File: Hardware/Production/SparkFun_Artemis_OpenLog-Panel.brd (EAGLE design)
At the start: 106.2 x 205 mm, 2031 parts, among them J100 CORTEX_JTAG, J107 MICRO-SD, J109 CORTEX_JTAG, J116 MICRO-SD, J118 CORTEX_JTAG, J125 MICRO-SD, J127 CORTEX_JTAG, J134 MICRO-SD, J14 CORTEX_JTAG, J17 MICRO-SD, J19 CORTEX_JTAG, J26 MICRO-SD, J28 CORTEX_JTAG, J35 MICRO-SD, J37 CORTEX_JTAG, J44 MICRO-SD, J46 CORTEX_JTAG, J53 MICRO-SD, J55 CORTEX_JTAG, J6 MICRO-SD, J62 MICRO-SD, J64 CORTEX_JTAG, J71 MICRO-SD, J73 CORTEX_JTAG, J8 CORTEX_JTAG, J80 MICRO-SD, J82 CORTEX_JTAG, J89 MICRO-SD, J91 CORTEX_JTAG, J98 MICRO-SD, Q1 20V/0.2A/8MHz/1.2Ω/1Vth, Q10 20V/0.2A/8MHz/1.2Ω/1Vth, Q11 20V/0.2A/8MHz/1.2Ω/1Vth, Q12 20V/4.2A/52mΩ/1.4W, Q13 20V/0.2A/8MHz/1.2Ω/1Vth, Q14 20V/0.2A/8MHz/1.2Ω/1Vth, Q15 20V/0.2A/8MHz/1.2Ω/1Vth, Q16 20V/0.2A/8MHz/1.2Ω/1Vth, Q17 20V/0.2A/8MHz/1.2Ω/1Vth, Q18 20V/4.2A/52mΩ/1.4W, Q19 20V/0.2A/8MHz/1.2Ω/1Vth, Q2 20V/4.2A/52mΩ/1.4W, Q20 20V/0.2A/8MHz/1.2Ω/1Vth, Q21 20V/0.2A/8MHz/1.2Ω/1Vth, Q22 20V/0.2A/8MHz/1.2Ω/1Vth, Q23 20V/0.2A/8MHz/1.2Ω/1Vth, Q24 20V/4.2A/52mΩ/1.4W, Q25 20V/0.2A/8MHz/1.2Ω/1Vth, Q26 20V/0.2A/8MHz/1.2Ω/1Vth, Q27 20V/0.2A/8MHz/1.2Ω/1Vth, Q28 20V/0.2A/8MHz/1.2Ω/1Vth, Q29 20V/0.2A/8MHz/1.2Ω/1Vth, Q3 20V/0.2A/8MHz/1.2Ω/1Vth, Q30 20V/4.2A/52mΩ/1.4W, Q31 20V/0.2A/8MHz/1.2Ω/1Vth, Q32 20V/0.2A/8MHz/1.2Ω/1Vth, Q33 20V/0.2A/8MHz/1.2Ω/1Vth, Q34 20V/0.2A/8MHz/1.2Ω/1Vth, Q35 20V/0.2A/8MHz/1.2Ω/1Vth, Q36 20V/4.2A/52mΩ/1.4W, Q37 20V/0.2A/8MHz/1.2Ω/1Vth, Q38 20V/0.2A/8MHz/1.2Ω/1Vth, Q39 20V/0.2A/8MHz/1.2Ω/1Vth, Q4 20V/0.2A/8MHz/1.2Ω/1Vth, Q40 20V/0.2A/8MHz/1.2Ω/1Vth, Q41 20V/0.2A/8MHz/1.2Ω/1Vth, Q42 20V/4.2A/52mΩ/1.4W, Q43 20V/0.2A/8MHz/1.2Ω/1Vth, Q44 20V/0.2A/8MHz/1.2Ω/1Vth, Q45 20V/0.2A/8MHz/1.2Ω/1Vth, Q46 20V/0.2A/8MHz/1.2Ω/1Vth, Q47 20V/0.2A/8MHz/1.2Ω/1Vth, Q48 20V/4.2A/52mΩ/1.4W, Q49 20V/0.2A/8MHz/1.2Ω/1Vth, Q5 20V/0.2A/8MHz/1.2Ω/1Vth, Q50 20V/0.2A/8MHz/1.2Ω/1Vth, Q51 20V/0.2A/8MHz/1.2Ω/1Vth, Q52 20V/0.2A/8MHz/1.2Ω/1Vth, Q53 20V/0.2A/8MHz/1.2Ω/1Vth, Q54 20V/4.2A/52mΩ/1.4W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

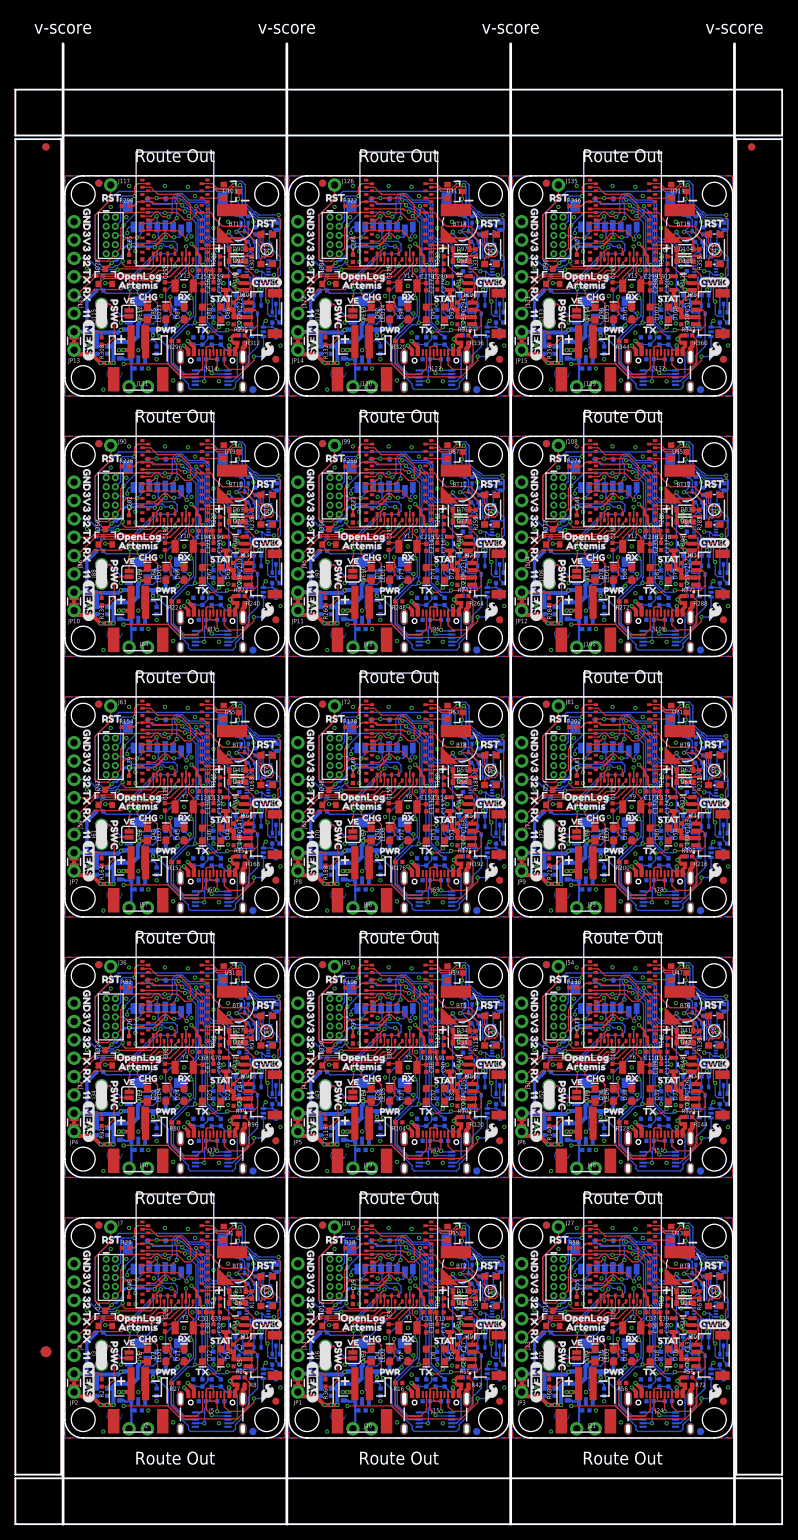
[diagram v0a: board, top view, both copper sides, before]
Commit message: Final V10 PCB tweaks!?
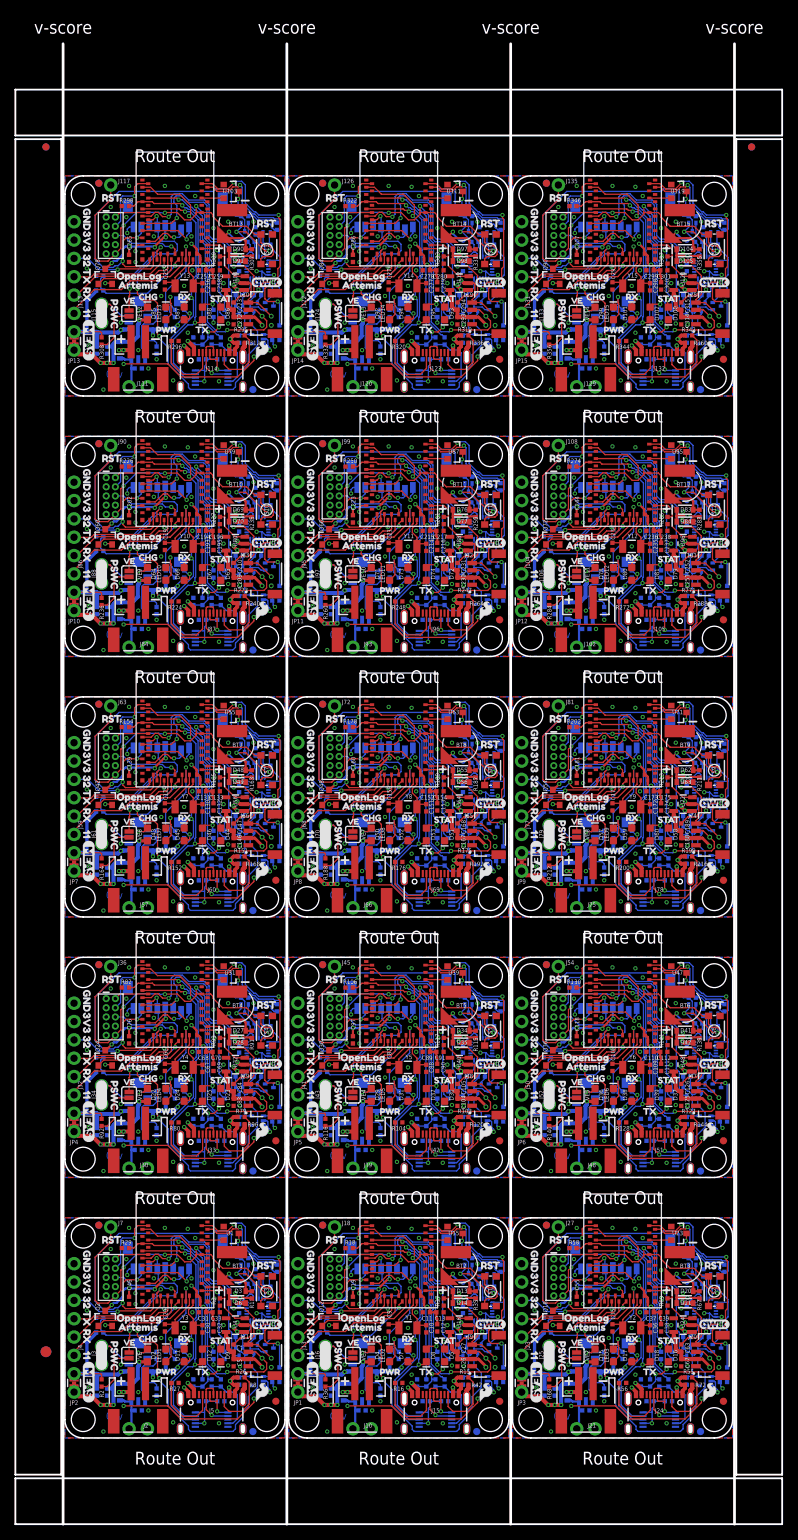
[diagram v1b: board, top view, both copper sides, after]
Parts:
- added GND, GND1, GND10, GND11, GND12, GND13, GND14, GND2, GND3, GND4, GND5, GND6, GND7, GND8, GND9, QWIIC_3.3V, QWIIC_3.3V1, QWIIC_3.3V10, QWIIC_3.3V11, QWIIC_3.3V12, QWIIC_3.3V13, QWIIC_3.3V14, QWIIC_3.3V2, QWIIC_3.3V3, QWIIC_3.3V4, QWIIC_3.3V5, QWIIC_3.3V6, QWIIC_3.3V7, QWIIC_3.3V8, QWIIC_3.3V9: TEST-POINTTP_15TH_THRU, SparkFun-Connectors:TP_15TH
- added U$586: (no value), buzzard_labels (14):322
- added U$587, U$588: (no value), buzzard_labels (14):GND5
- added U$589, U$590: (no value), buzzard_labels (14):RX1
- added U$591, U$592: (no value), buzzard_labels (14):TX0
- added U$593, U$594: (no value), buzzard_labels:PSWC0
- added U$595: (no value), buzzard_labels (19):VE0
- added U$596, U$597: (no value), RST_04:RST0
- added U$598: (no value), output:C0
- added U$599: (no value), output:D0
- added U$600: (no value), output:30
- SCL, SCL1, SCL10, SCL11, SCL12, SCL13, SCL14, SCL2, SCL3, SCL4, SCL5, SCL6, SCL7, SCL8, SCL9, SDA, SDA1, SDA10, SDA11, SDA12, SDA13, SDA14, SDA2, SDA3, SDA4, SDA5, SDA6, SDA7, SDA8, SDA9: value TEST-POINT3 -> TEST-POINTTP_15TH_THRU; device SparkFun-Connectors:PAD.03X.03 -> SparkFun-Connectors:TP_15TH
- U$100, U$60: device buzzard_labels (14):3V34 -> buzzard_labels (13):VIN8
- U$101, U$102, U$141, U$62: device buzzard_labels (14):113 -> buzzard_labels (14):3V34
- U$103, U$104, U$143, U$64: device buzzard_labels (14):322 -> buzzard_labels (14):113
- U$105, U$106, U$145, U$66: device buzzard_labels (14):GND5 -> buzzard_labels (14):322
- U$107, U$108, U$147, U$68: device buzzard_labels (14):RX1 -> buzzard_labels (14):GND5
- U$109, U$110, U$149, U$70: device buzzard_labels (14):TX0 -> buzzard_labels (14):RX1
- U$111, U$112, U$151, U$72: device buzzard_labels:PSWC0 -> buzzard_labels (14):TX0
- U$113, U$74: device buzzard_labels (19):VE0 -> buzzard_labels:PSWC0
- U$114, U$153, U$154, U$193: device RST_04:RST0 -> buzzard_labels:PSWC0
- U$115, U$75: device RST_04:RST0 -> buzzard_labels (19):VE0
- U$116, U$77: device output:C0 -> RST_04:RST0
- U$117, U$156: device output:D0 -> RST_04:RST0
- U$118: device buzzard_labels (2):MEAS3 -> output:C0
- U$119, U$359: device buzzard_labels (1):X0 -> output:D0
- U$120, U$360: device buzzard_labels (1):Y1 -> output:30
- U$121, U$361: device buzzard_labels (1):Z2 -> buzzard_labels (2):MEAS3
- U$122: device buzzard_labels (1):G5 -> buzzard_labels (1):X0
- U$123: device buzzard_labels (1):A4 -> buzzard_labels (1):Y1
- U$124: device buzzard_labels (1):M3 -> buzzard_labels (1):Z2
- U$125: device buzzard_labels (1):X0 -> buzzard_labels (1):G5
- U$126: device buzzard_labels (1):Y1 -> buzzard_labels (1):A4
- U$127: device buzzard_labels (1):Z2 -> buzzard_labels (1):M3
- U$128, U$362: device qwiic#logo#jpg:QWIIC#LOGO#JPG -> buzzard_labels (1):X0
- U$129, U$363: device buzzard_labels (12):CHG2 -> buzzard_labels (1):Y1
- U$130, U$364: device buzzard_labels (12):PWR0 -> buzzard_labels (1):Z2
- U$131: device buzzard_labels (12):RX4 -> qwiic#logo#jpg:QWIIC#LOGO#JPG
- U$132: device buzzard_labels (12):STAT5 -> buzzard_labels (12):CHG2
- U$133: device buzzard_labels (12):TX3 -> buzzard_labels (12):PWR0
- U$134: device buzzard_labels (13):ARTEMIS13 -> buzzard_labels (12):RX4
- U$135: device buzzard_labels (13):OPENLOG12 -> buzzard_labels (12):STAT5
- U$136: device buzzard_labels (13):RST9 -> buzzard_labels (12):TX3
- U$137: device buzzard_labels (13):VIN8 -> buzzard_labels (13):ARTEMIS13
- U$138, U$178: device buzzard_labels (14):3V34 -> buzzard_labels (13):OPENLOG12
- U$139, U$99: device buzzard_labels (14):3V34 -> buzzard_labels (13):RST9
- U$140, U$180: device buzzard_labels (14):113 -> buzzard_labels (13):VIN8
- U$142, U$181, U$182, U$221: device buzzard_labels (14):322 -> buzzard_labels (14):3V34
- U$144, U$183, U$184, U$223: device buzzard_labels (14):GND5 -> buzzard_labels (14):113
- U$146, U$185, U$186, U$225: device buzzard_labels (14):RX1 -> buzzard_labels (14):322
- U$148, U$187, U$188, U$227: device buzzard_labels (14):TX0 -> buzzard_labels (14):GND5
- U$15: device buzzard_labels (2):MEAS3 -> output:30
- U$150, U$189, U$190, U$229: device buzzard_labels:PSWC0 -> buzzard_labels (14):RX1
- U$152, U$191: device buzzard_labels (19):VE0 -> buzzard_labels (14):TX0
- U$155: device output:C0 -> buzzard_labels (19):VE0
- U$157, U$196: device buzzard_labels (2):MEAS3 -> RST_04:RST0
- U$158, U$398: device buzzard_labels (1):X0 -> output:C0
- U$159, U$399: device buzzard_labels (1):Y1 -> output:D0
- U$16, U$281: device buzzard_labels (1):X0 -> buzzard_labels (2):MEAS3
- U$160, U$400: device buzzard_labels (1):Z2 -> output:30
- U$161: device buzzard_labels (1):G5 -> buzzard_labels (2):MEAS3
- U$162: device buzzard_labels (1):A4 -> buzzard_labels (1):X0
- U$163: device buzzard_labels (1):M3 -> buzzard_labels (1):Y1
- U$164: device buzzard_labels (1):X0 -> buzzard_labels (1):Z2
- U$165: device buzzard_labels (1):Y1 -> buzzard_labels (1):G5
- U$166: device buzzard_labels (1):Z2 -> buzzard_labels (1):A4
- U$167: device qwiic#logo#jpg:QWIIC#LOGO#JPG -> buzzard_labels (1):M3
- U$168, U$402: device buzzard_labels (12):CHG2 -> buzzard_labels (1):X0
- U$169, U$403: device buzzard_labels (12):PWR0 -> buzzard_labels (1):Y1
- U$17, U$23, U$282: device buzzard_labels (1):Y1 -> buzzard_labels (1):X0
- U$170, U$404: device buzzard_labels (12):RX4 -> buzzard_labels (1):Z2
- U$171: device buzzard_labels (12):STAT5 -> qwiic#logo#jpg:QWIIC#LOGO#JPG
- U$172: device buzzard_labels (12):TX3 -> buzzard_labels (12):CHG2
- U$173: device buzzard_labels (13):ARTEMIS13 -> buzzard_labels (12):PWR0
- U$174: device buzzard_labels (13):OPENLOG12 -> buzzard_labels (12):RX4
- U$175: device buzzard_labels (13):RST9 -> buzzard_labels (12):STAT5
- U$176: device buzzard_labels (13):VIN8 -> buzzard_labels (12):TX3
- U$177, U$217: device buzzard_labels (14):3V34 -> buzzard_labels (13):ARTEMIS13
- U$179, U$219: device buzzard_labels (14):113 -> buzzard_labels (13):RST9
- U$18, U$24, U$283: device buzzard_labels (1):Z2 -> buzzard_labels (1):Y1
- U$19: device buzzard_labels (1):G5 -> buzzard_labels (1):Z2
- U$192, U$231, U$232, U$271: device RST_04:RST0 -> buzzard_labels (14):TX0
- U$194, U$233: device output:C0 -> buzzard_labels:PSWC0
- U$195: device output:D0 -> buzzard_labels (19):VE0
- U$197, U$236, U$437, U$476: device buzzard_labels (1):X0 -> RST_04:RST0
- U$198, U$438: device buzzard_labels (1):Y1 -> output:C0
- U$199, U$439: device buzzard_labels (1):Z2 -> output:D0
- U$20: device buzzard_labels (1):A4 -> buzzard_labels (1):G5
- U$200: device buzzard_labels (1):G5 -> output:30
- U$201: device buzzard_labels (1):A4 -> buzzard_labels (2):MEAS3
- U$202: device buzzard_labels (1):M3 -> buzzard_labels (1):X0
- U$203: device buzzard_labels (1):X0 -> buzzard_labels (1):Y1
- U$204: device buzzard_labels (1):Y1 -> buzzard_labels (1):Z2
- U$205: device buzzard_labels (1):Z2 -> buzzard_labels (1):G5
- U$206: device qwiic#logo#jpg:QWIIC#LOGO#JPG -> buzzard_labels (1):A4
- U$207: device buzzard_labels (12):CHG2 -> buzzard_labels (1):M3
- U$208, U$442: device buzzard_labels (12):PWR0 -> buzzard_labels (1):X0
- U$209, U$443: device buzzard_labels (12):RX4 -> buzzard_labels (1):Y1
- U$21: device buzzard_labels (1):M3 -> buzzard_labels (1):A4
- U$210, U$444: device buzzard_labels (12):STAT5 -> buzzard_labels (1):Z2
- U$211: device buzzard_labels (12):TX3 -> qwiic#logo#jpg:QWIIC#LOGO#JPG
- U$212: device buzzard_labels (13):ARTEMIS13 -> buzzard_labels (12):CHG2
- U$213: device buzzard_labels (13):OPENLOG12 -> buzzard_labels (12):PWR0
- U$214: device buzzard_labels (13):RST9 -> buzzard_labels (12):RX4
- U$215: device buzzard_labels (13):VIN8 -> buzzard_labels (12):STAT5
- U$216, U$256: device buzzard_labels (14):3V34 -> buzzard_labels (12):TX3
- U$218, U$258: device buzzard_labels (14):113 -> buzzard_labels (13):OPENLOG12
- U$22: device buzzard_labels (1):X0 -> buzzard_labels (1):M3
- U$220, U$260: device buzzard_labels (14):322 -> buzzard_labels (13):VIN8
- U$222, U$261, U$262, U$301: device buzzard_labels (14):GND5 -> buzzard_labels (14):3V34
- U$224, U$263, U$264, U$303: device buzzard_labels (14):RX1 -> buzzard_labels (14):113
- U$226, U$265, U$266, U$305: device buzzard_labels (14):TX0 -> buzzard_labels (14):322
- U$228, U$267, U$268, U$307: device buzzard_labels:PSWC0 -> buzzard_labels (14):GND5
- U$230, U$269: device buzzard_labels (19):VE0 -> buzzard_labels (14):RX1
- U$234, U$273: device output:D0 -> buzzard_labels:PSWC0
- U$235: device buzzard_labels (2):MEAS3 -> buzzard_labels (19):VE0
- U$237, U$276, U$477, U$516: device buzzard_labels (1):Y1 -> RST_04:RST0
- U$238, U$478: device buzzard_labels (1):Z2 -> output:C0
- U$239: device buzzard_labels (1):G5 -> output:D0
- U$240: device buzzard_labels (1):A4 -> output:30
- U$241: device buzzard_labels (1):M3 -> buzzard_labels (2):MEAS3
- U$245: device qwiic#logo#jpg:QWIIC#LOGO#JPG -> buzzard_labels (1):G5
- U$246: device buzzard_labels (12):CHG2 -> buzzard_labels (1):A4
- U$247: device buzzard_labels (12):PWR0 -> buzzard_labels (1):M3
- U$248, U$482: device buzzard_labels (12):RX4 -> buzzard_labels (1):X0
- U$249, U$483: device buzzard_labels (12):STAT5 -> buzzard_labels (1):Y1
- U$25, U$284: device qwiic#logo#jpg:QWIIC#LOGO#JPG -> buzzard_labels (1):Z2
- U$250, U$484: device buzzard_labels (12):TX3 -> buzzard_labels (1):Z2
- U$251: device buzzard_labels (13):ARTEMIS13 -> qwiic#logo#jpg:QWIIC#LOGO#JPG
- U$252: device buzzard_labels (13):OPENLOG12 -> buzzard_labels (12):CHG2
- U$253: device buzzard_labels (13):RST9 -> buzzard_labels (12):PWR0
- U$254: device buzzard_labels (13):VIN8 -> buzzard_labels (12):RX4
- U$255, U$295: device buzzard_labels (14):3V34 -> buzzard_labels (12):STAT5
- U$257, U$297: device buzzard_labels (14):113 -> buzzard_labels (13):ARTEMIS13
- U$259, U$299: device buzzard_labels (14):322 -> buzzard_labels (13):RST9
- U$26: device buzzard_labels (12):CHG2 -> qwiic#logo#jpg:QWIIC#LOGO#JPG
- U$270, U$309, U$310, U$349: device RST_04:RST0 -> buzzard_labels (14):RX1
- U$272, U$311: device output:C0 -> buzzard_labels (14):TX0
- U$274, U$313: device buzzard_labels (2):MEAS3 -> buzzard_labels:PSWC0
- U$275, U$515: device buzzard_labels (1):X0 -> buzzard_labels (19):VE0
- U$277, U$316, U$517, U$556: device buzzard_labels (1):Z2 -> RST_04:RST0
- U$278: device buzzard_labels (1):G5 -> output:C0
- U$279: device buzzard_labels (1):A4 -> output:D0
- U$280: device buzzard_labels (1):M3 -> output:30
- U$285: device buzzard_labels (12):CHG2 -> buzzard_labels (1):G5
- U$286: device buzzard_labels (12):PWR0 -> buzzard_labels (1):A4
- U$287: device buzzard_labels (12):RX4 -> buzzard_labels (1):M3
- U$288, U$522: device buzzard_labels (12):STAT5 -> buzzard_labels (1):X0
- U$289, U$523: device buzzard_labels (12):TX3 -> buzzard_labels (1):Y1
- U$29: device buzzard_labels (12):PWR0 -> buzzard_labels (12):CHG2
- U$290, U$524: device buzzard_labels (13):ARTEMIS13 -> buzzard_labels (1):Z2
- U$291: device buzzard_labels (13):OPENLOG12 -> qwiic#logo#jpg:QWIIC#LOGO#JPG
- U$292: device buzzard_labels (13):RST9 -> buzzard_labels (12):CHG2
- U$293: device buzzard_labels (13):VIN8 -> buzzard_labels (12):PWR0
- U$294, U$334: device buzzard_labels (14):3V34 -> buzzard_labels (12):RX4
- U$296, U$336: device buzzard_labels (14):113 -> buzzard_labels (12):TX3
- U$298, U$338: device buzzard_labels (14):322 -> buzzard_labels (13):OPENLOG12
- U$30: device buzzard_labels (12):RX4 -> buzzard_labels (12):PWR0
- U$300, U$340: device buzzard_labels (14):GND5 -> buzzard_labels (13):VIN8
- U$302, U$341, U$342, U$381: device buzzard_labels (14):RX1 -> buzzard_labels (14):3V34
- U$304, U$343, U$344, U$383: device buzzard_labels (14):TX0 -> buzzard_labels (14):113
- U$306, U$345, U$346, U$385: device buzzard_labels:PSWC0 -> buzzard_labels (14):322
- U$308, U$347: device buzzard_labels (19):VE0 -> buzzard_labels (14):GND5
- U$31: device buzzard_labels (12):STAT5 -> buzzard_labels (12):RX4
- U$312, U$351: device output:D0 -> buzzard_labels (14):TX0
- U$314, U$353, U$554: device buzzard_labels (1):X0 -> buzzard_labels:PSWC0
- U$315, U$555: device buzzard_labels (1):Y1 -> buzzard_labels (19):VE0
- U$317, U$356: device buzzard_labels (1):G5 -> RST_04:RST0
- U$318: device buzzard_labels (1):A4 -> output:C0
- U$319: device buzzard_labels (1):M3 -> output:D0
- U$320, U$80: device buzzard_labels (1):X0 -> output:30
- U$321, U$81: device buzzard_labels (1):Y1 -> buzzard_labels (2):MEAS3
- U$322, U$82, U$88: device buzzard_labels (1):Z2 -> buzzard_labels (1):X0
- U$323, U$89: device qwiic#logo#jpg:QWIIC#LOGO#JPG -> buzzard_labels (1):Y1
- U$324, U$90: device buzzard_labels (12):CHG2 -> buzzard_labels (1):Z2
- U$325: device buzzard_labels (12):PWR0 -> buzzard_labels (1):G5
- U$326: device buzzard_labels (12):RX4 -> buzzard_labels (1):A4
- U$327: device buzzard_labels (12):STAT5 -> buzzard_labels (1):M3
- U$328, U$562: device buzzard_labels (12):TX3 -> buzzard_labels (1):X0
- U$329, U$563: device buzzard_labels (13):ARTEMIS13 -> buzzard_labels (1):Y1
- U$330, U$564: device buzzard_labels (13):OPENLOG12 -> buzzard_labels (1):Z2
- U$331: device buzzard_labels (13):RST9 -> qwiic#logo#jpg:QWIIC#LOGO#JPG
- U$332: device buzzard_labels (13):VIN8 -> buzzard_labels (12):CHG2
- U$333, U$373: device buzzard_labels (14):3V34 -> buzzard_labels (12):PWR0
- U$335, U$375: device buzzard_labels (14):113 -> buzzard_labels (12):STAT5
- U$337, U$377: device buzzard_labels (14):322 -> buzzard_labels (13):ARTEMIS13
- U$339, U$379: device buzzard_labels (14):GND5 -> buzzard_labels (13):RST9
- U$348, U$387, U$388, U$427: device RST_04:RST0 -> buzzard_labels (14):GND5
- U$350, U$389: device output:C0 -> buzzard_labels (14):RX1
- U$352, U$391: device buzzard_labels (2):MEAS3 -> buzzard_labels (14):TX0
- U$354, U$393: device buzzard_labels (1):Y1 -> buzzard_labels:PSWC0
- U$355: device buzzard_labels (1):Z2 -> buzzard_labels (19):VE0
- U$357, U$396: device buzzard_labels (1):A4 -> RST_04:RST0
- U$358: device buzzard_labels (1):M3 -> output:C0
- U$365: device buzzard_labels (12):RX4 -> buzzard_labels (1):G5
- U$366: device buzzard_labels (12):STAT5 -> buzzard_labels (1):A4
- U$367: device buzzard_labels (12):TX3 -> buzzard_labels (1):M3
- U$368: device buzzard_labels (13):ARTEMIS13 -> buzzard_labels (1):X0
- U$369: device buzzard_labels (13):OPENLOG12 -> buzzard_labels (1):Y1
- U$370: device buzzard_labels (13):RST9 -> buzzard_labels (1):Z2
- U$371: device buzzard_labels (13):VIN8 -> qwiic#logo#jpg:QWIIC#LOGO#JPG
- U$372, U$412: device buzzard_labels (14):3V34 -> buzzard_labels (12):CHG2
- U$374, U$414: device buzzard_labels (14):113 -> buzzard_labels (12):RX4
- U$376, U$416: device buzzard_labels (14):322 -> buzzard_labels (12):TX3
- U$378, U$418: device buzzard_labels (14):GND5 -> buzzard_labels (13):OPENLOG12
- U$380, U$420: device buzzard_labels (14):RX1 -> buzzard_labels (13):VIN8
- U$382, U$421, U$422, U$461: device buzzard_labels (14):TX0 -> buzzard_labels (14):3V34
- U$384, U$423, U$424, U$463: device buzzard_labels:PSWC0 -> buzzard_labels (14):113
- U$386, U$425: device buzzard_labels (19):VE0 -> buzzard_labels (14):322
- U$390, U$429: device output:D0 -> buzzard_labels (14):RX1
- U$392, U$431: device buzzard_labels (1):X0 -> buzzard_labels (14):TX0
- U$394, U$433: device buzzard_labels (1):Z2 -> buzzard_labels:PSWC0
- U$395: device buzzard_labels (1):G5 -> buzzard_labels (19):VE0
- U$397, U$436: device buzzard_labels (1):M3 -> RST_04:RST0
- U$401: device qwiic#logo#jpg:QWIIC#LOGO#JPG -> buzzard_labels (2):MEAS3
- U$405: device buzzard_labels (12):STAT5 -> buzzard_labels (1):G5
- U$406: device buzzard_labels (12):TX3 -> buzzard_labels (1):A4
- U$407: device buzzard_labels (13):ARTEMIS13 -> buzzard_labels (1):M3
- U$408: device buzzard_labels (13):OPENLOG12 -> buzzard_labels (1):X0
- U$409: device buzzard_labels (13):RST9 -> buzzard_labels (1):Y1
- U$410: device buzzard_labels (13):VIN8 -> buzzard_labels (1):Z2
- U$411, U$451: device buzzard_labels (14):3V34 -> qwiic#logo#jpg:QWIIC#LOGO#JPG
- U$413, U$453: device buzzard_labels (14):113 -> buzzard_labels (12):PWR0
- U$415, U$455: device buzzard_labels (14):322 -> buzzard_labels (12):STAT5
- U$417, U$457: device buzzard_labels (14):GND5 -> buzzard_labels (13):ARTEMIS13
- U$419, U$459: device buzzard_labels (14):RX1 -> buzzard_labels (13):RST9
- U$426, U$465, U$466, U$505: device RST_04:RST0 -> buzzard_labels (14):322
- U$428, U$467: device output:C0 -> buzzard_labels (14):GND5
- U$430, U$469: device buzzard_labels (2):MEAS3 -> buzzard_labels (14):RX1
- U$432, U$471: device buzzard_labels (1):Y1 -> buzzard_labels (14):TX0
- U$434, U$473: device buzzard_labels (1):G5 -> buzzard_labels:PSWC0
- U$435: device buzzard_labels (1):A4 -> buzzard_labels (19):VE0
- U$440: device qwiic#logo#jpg:QWIIC#LOGO#JPG -> output:30
- U$441: device buzzard_labels (12):CHG2 -> buzzard_labels (2):MEAS3
- U$445: device buzzard_labels (12):TX3 -> buzzard_labels (1):G5
- U$446: device buzzard_labels (13):ARTEMIS13 -> buzzard_labels (1):A4
- U$447: device buzzard_labels (13):OPENLOG12 -> buzzard_labels (1):M3
- U$448: device buzzard_labels (13):RST9 -> buzzard_labels (1):X0
- U$449: device buzzard_labels (13):VIN8 -> buzzard_labels (1):Y1
- U$450, U$490: device buzzard_labels (14):3V34 -> buzzard_labels (1):Z2
- U$452, U$492: device buzzard_labels (14):113 -> buzzard_labels (12):CHG2
- U$454, U$494: device buzzard_labels (14):322 -> buzzard_labels (12):RX4
- U$456, U$496: device buzzard_labels (14):GND5 -> buzzard_labels (12):TX3
- U$458, U$498: device buzzard_labels (14):RX1 -> buzzard_labels (13):OPENLOG12
- U$460, U$500: device buzzard_labels (14):TX0 -> buzzard_labels (13):VIN8
- U$462, U$501, U$502, U$541: device buzzard_labels:PSWC0 -> buzzard_labels (14):3V34
- U$464, U$503: device buzzard_labels (19):VE0 -> buzzard_labels (14):113
- U$468, U$507: device output:D0 -> buzzard_labels (14):GND5
- U$470, U$509: device buzzard_labels (1):X0 -> buzzard_labels (14):RX1
- U$472, U$511: device buzzard_labels (1):Z2 -> buzzard_labels (14):TX0
- U$474, U$513: device buzzard_labels (1):A4 -> buzzard_labels:PSWC0
- U$475: device buzzard_labels (1):M3 -> buzzard_labels (19):VE0
- U$479: device qwiic#logo#jpg:QWIIC#LOGO#JPG -> output:D0
- U$480: device buzzard_labels (12):CHG2 -> output:30
- U$481: device buzzard_labels (12):PWR0 -> buzzard_labels (2):MEAS3
- U$485: device buzzard_labels (13):ARTEMIS13 -> buzzard_labels (1):G5
- U$486: device buzzard_labels (13):OPENLOG12 -> buzzard_labels (1):A4
- U$487: device buzzard_labels (13):RST9 -> buzzard_labels (1):M3
- U$488: device buzzard_labels (13):VIN8 -> buzzard_labels (1):X0
- U$489, U$529: device buzzard_labels (14):3V34 -> buzzard_labels (1):Y1
- U$491, U$531: device buzzard_labels (14):113 -> qwiic#logo#jpg:QWIIC#LOGO#JPG
- U$493, U$533: device buzzard_labels (14):322 -> buzzard_labels (12):PWR0
- U$495, U$535: device buzzard_labels (14):GND5 -> buzzard_labels (12):STAT5
- U$497, U$537: device buzzard_labels (14):RX1 -> buzzard_labels (13):ARTEMIS13
- U$499, U$539: device buzzard_labels (14):TX0 -> buzzard_labels (13):RST9
- U$504, U$543, U$544, U$583: device RST_04:RST0 -> buzzard_labels (14):113
- U$506, U$545: device output:C0 -> buzzard_labels (14):322
- U$508, U$547: device buzzard_labels (2):MEAS3 -> buzzard_labels (14):GND5
- U$510, U$549: device buzzard_labels (1):Y1 -> buzzard_labels (14):RX1
- U$512, U$551: device buzzard_labels (1):G5 -> buzzard_labels (14):TX0
- U$514, U$553: device buzzard_labels (1):M3 -> buzzard_labels:PSWC0
- U$518: device qwiic#logo#jpg:QWIIC#LOGO#JPG -> output:C0
- U$519: device buzzard_labels (12):CHG2 -> output:D0
- U$52: device buzzard_labels (12):TX3 -> buzzard_labels (12):STAT5
- U$520: device buzzard_labels (12):PWR0 -> output:30
- U$521: device buzzard_labels (12):RX4 -> buzzard_labels (2):MEAS3
- U$525: device buzzard_labels (13):OPENLOG12 -> buzzard_labels (1):G5
- U$526: device buzzard_labels (13):RST9 -> buzzard_labels (1):A4
- U$527: device buzzard_labels (13):VIN8 -> buzzard_labels (1):M3
- U$528, U$568: device buzzard_labels (14):3V34 -> buzzard_labels (1):X0
- U$53: device buzzard_labels (13):ARTEMIS13 -> buzzard_labels (12):TX3
- U$530, U$570: device buzzard_labels (14):113 -> buzzard_labels (1):Z2
- U$532, U$572: device buzzard_labels (14):322 -> buzzard_labels (12):CHG2
- U$534, U$574: device buzzard_labels (14):GND5 -> buzzard_labels (12):RX4
- U$536, U$576: device buzzard_labels (14):RX1 -> buzzard_labels (12):TX3
- U$538, U$578: device buzzard_labels (14):TX0 -> buzzard_labels (13):OPENLOG12
- U$540, U$580: device buzzard_labels:PSWC0 -> buzzard_labels (13):VIN8
- U$542, U$581: device buzzard_labels (19):VE0 -> buzzard_labels (14):3V34
- U$546, U$585: device output:D0 -> buzzard_labels (14):322
- U$548: device buzzard_labels (1):X0 -> buzzard_labels (14):GND5
- U$550: device buzzard_labels (1):Z2 -> buzzard_labels (14):RX1
- U$552: device buzzard_labels (1):A4 -> buzzard_labels (14):TX0
- U$557: device qwiic#logo#jpg:QWIIC#LOGO#JPG -> RST_04:RST0
- U$558: device buzzard_labels (12):CHG2 -> output:C0
- U$559: device buzzard_labels (12):PWR0 -> output:D0
- U$560: device buzzard_labels (12):RX4 -> output:30
- U$561: device buzzard_labels (12):STAT5 -> buzzard_labels (2):MEAS3
- U$565: device buzzard_labels (13):RST9 -> buzzard_labels (1):G5
- U$566: device buzzard_labels (13):VIN8 -> buzzard_labels (1):A4
- U$567: device buzzard_labels (14):3V34 -> buzzard_labels (1):M3
- U$569: device buzzard_labels (14):113 -> buzzard_labels (1):Y1
- U$57: device buzzard_labels (13):OPENLOG12 -> buzzard_labels (13):ARTEMIS13
- U$571: device buzzard_labels (14):322 -> qwiic#logo#jpg:QWIIC#LOGO#JPG
- U$573: device buzzard_labels (14):GND5 -> buzzard_labels (12):PWR0
- U$575: device buzzard_labels (14):RX1 -> buzzard_labels (12):STAT5
- U$577: device buzzard_labels (14):TX0 -> buzzard_labels (13):ARTEMIS13
- U$579: device buzzard_labels:PSWC0 -> buzzard_labels (13):RST9
- U$58: device buzzard_labels (13):RST9 -> buzzard_labels (13):OPENLOG12
- U$582: device RST_04:RST0 -> buzzard_labels (14):3V34
- U$584: device output:C0 -> buzzard_labels (14):113
- U$59: device buzzard_labels (13):VIN8 -> buzzard_labels (13):RST9
- U$78: device output:D0 -> output:C0
- U$79: device buzzard_labels (2):MEAS3 -> output:D0
- U$83: device buzzard_labels (1):G5 -> buzzard_labels (1):Y1
- U$84: device buzzard_labels (1):A4 -> buzzard_labels (1):Z2
- U$85: device buzzard_labels (1):M3 -> buzzard_labels (1):G5
- U$86: device buzzard_labels (1):X0 -> buzzard_labels (1):A4
- U$87: device buzzard_labels (1):Y1 -> buzzard_labels (1):M3
- U$91: device buzzard_labels (12):PWR0 -> qwiic#logo#jpg:QWIIC#LOGO#JPG
- U$92: device buzzard_labels (12):RX4 -> buzzard_labels (12):CHG2
- U$93: device buzzard_labels (12):STAT5 -> buzzard_labels (12):PWR0
- U$94: device buzzard_labels (12):TX3 -> buzzard_labels (12):RX4
- U$95: device buzzard_labels (13):ARTEMIS13 -> buzzard_labels (12):STAT5
- U$96: device buzzard_labels (13):OPENLOG12 -> buzzard_labels (12):TX3
- U$97: device buzzard_labels (13):RST9 -> buzzard_labels (13):ARTEMIS13
- U$98: device buzzard_labels (13):VIN8 -> buzzard_labels (13):OPENLOG12
- U100, U108, U116, U13, U20, U28, U36, U44, U52, U60, U68, U76, U84, U9, U92: value ICM-20948 -> 9DoF IMU; device SparkFun-Sensors:QFN24-3X3 -> SparkFun-Sensors:QFN24-3X3-ICM-20948
- U102, U104, U110, U112, U118, U12, U120, U16, U22, U24, U3, U30, U32, U38, U4, U40, U46, U48, U54, U56, U62, U64, U70, U72, U78, U80, U86, U88, U94, U96: value AP2112K -> 3.3V
- moved U$118 95.0 mm to (91.3, 11.0), flipped to the bottom, turned to 0 degrees
- moved U$480 88.5 mm to (88.4, 118.0), flipped to the bottom
- moved U$238 88.2 mm to (91.3, 47.1)
- moved U$120 83.6 mm to (88.4, 9.78)
- moved U$119 83.2 mm to (88.4, 10.9), turned to 0 degrees
- moved U$239 80.3 mm to (88.4, 47.0)
- moved U$240 80.2 mm to (88.4, 45.8)
- moved U$235 74.1 mm to (69.3, 49.3), turned to 0 degrees
- moved U$479 73.0 mm to (88.4, 119.1), flipped to the bottom
- moved U$358 71.8 mm to (91.3, 83.2)
- moved U$353 71.0 mm to (68.8, 80.5), turned to 90 degrees
- moved U$355 70.7 mm to (69.3, 85.3), flipped to the top
- moved U$352 69.6 mm to (65.0, 86.7), flipped to the bottom, turned to 90 degrees
- moved U$360 69.2 mm to (88.4, 81.9)
- moved U$469 69.0 mm to (65.0, 124.2)
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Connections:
- net ICM-20948-LV_MISO renamed ICM-20948-LV_SDO
- net ICM-20948-LV_MISO1 renamed ICM-20948-LV_SDO1
- net ICM-20948-LV_MISO10 renamed ICM-20948-LV_SDO10
- net ICM-20948-LV_MISO11 renamed ICM-20948-LV_SDO11
- net ICM-20948-LV_MISO12 renamed ICM-20948-LV_SDO12
- net ICM-20948-LV_MISO13 renamed ICM-20948-LV_SDO13
- net ICM-20948-LV_MISO14 renamed ICM-20948-LV_SDO14
- net ICM-20948-LV_MISO2 renamed ICM-20948-LV_SDO2
- net ICM-20948-LV_MISO3 renamed ICM-20948-LV_SDO3
- net ICM-20948-LV_MISO4 renamed ICM-20948-LV_SDO4
- net ICM-20948-LV_MISO5 renamed ICM-20948-LV_SDO5
- net ICM-20948-LV_MISO6 renamed ICM-20948-LV_SDO6
- net ICM-20948-LV_MISO7 renamed ICM-20948-LV_SDO7
- net ICM-20948-LV_MISO8 renamed ICM-20948-LV_SDO8
- net ICM-20948-LV_MISO9 renamed ICM-20948-LV_SDO9
- net ICM-20948-LV_MOSI renamed ICM-20948-LV_SDI
- net ICM-20948-LV_MOSI1 renamed ICM-20948-LV_SDI1
- net ICM-20948-LV_MOSI10 renamed ICM-20948-LV_SDI10
- net ICM-20948-LV_MOSI11 renamed ICM-20948-LV_SDI11
- net ICM-20948-LV_MOSI12 renamed ICM-20948-LV_SDI12
- net ICM-20948-LV_MOSI13 renamed ICM-20948-LV_SDI13
- net ICM-20948-LV_MOSI14 renamed ICM-20948-LV_SDI14
- net ICM-20948-LV_MOSI2 renamed ICM-20948-LV_SDI2
- net ICM-20948-LV_MOSI3 renamed ICM-20948-LV_SDI3
- net ICM-20948-LV_MOSI4 renamed ICM-20948-LV_SDI4
- net ICM-20948-LV_MOSI5 renamed ICM-20948-LV_SDI5
- net ICM-20948-LV_MOSI6 renamed ICM-20948-LV_SDI6
- net ICM-20948-LV_MOSI7 renamed ICM-20948-LV_SDI7
- net ICM-20948-LV_MOSI8 renamed ICM-20948-LV_SDI8
- net ICM-20948-LV_MOSI9 renamed ICM-20948-LV_SDI9
- removed net MISO: J6.DO, Q10.3, R49.1, U8.~D22, U8.~D6
- removed net MISO1: J17.DO, Q11.3, R34.1, U6.~D22, U6.~D6
- removed net MISO10: J98.DO, Q65.3, R258.1, U82.~D22, U82.~D6
- removed net MISO11: J107.DO, Q71.3, R282.1, U90.~D22, U90.~D6
- removed net MISO12: J116.DO, Q77.3, R306.1, U98.~D22, U98.~D6
- removed net MISO13: J125.DO, Q83.3, R330.1, U106.~D22, U106.~D6
- removed net MISO14: J134.DO, Q89.3, R354.1, U114.~D22, U114.~D6
- removed net MISO2: J26.DO, Q17.3, R66.1, U18.~D22, U18.~D6
- removed net MISO3: J35.DO, Q23.3, R90.1, U26.~D22, U26.~D6
- removed net MISO4: J44.DO, Q29.3, R114.1, U34.~D22, U34.~D6
- removed net MISO5: J53.DO, Q35.3, R138.1, U42.~D22, U42.~D6
- removed net MISO6: J62.DO, Q41.3, R162.1, U50.~D22, U50.~D6
- removed net MISO7: J71.DO, Q47.3, R186.1, U58.~D22, U58.~D6
- removed net MISO8: J80.DO, Q53.3, R210.1, U66.~D22, U66.~D6
- removed net MISO9: J89.DO, Q59.3, R234.1, U74.~D22, U74.~D6
- removed net MOSI: J6.DI, Q3.3, U8.D7
- removed net MOSI1: J17.DI, Q5.3, U6.D7
- removed net MOSI10: J98.DI, Q62.3, U82.D7
- removed net MOSI11: J107.DI, Q68.3, U90.D7
- removed net MOSI12: J116.DI, Q74.3, U98.D7
- removed net MOSI13: J125.DI, Q80.3, U106.D7
- removed net MOSI14: J134.DI, Q86.3, U114.D7
- removed net MOSI2: J26.DI, Q14.3, U18.D7
- removed net MOSI3: J35.DI, Q20.3, U26.D7
- removed net MOSI4: J44.DI, Q26.3, U34.D7
- removed net MOSI5: J53.DI, Q32.3, U42.D7
- removed net MOSI6: J62.DI, Q38.3, U50.D7
- removed net MOSI7: J71.DI, Q44.3, U58.D7
- removed net MOSI8: J80.DI, Q50.3, U66.D7
- removed net MOSI9: J89.DI, Q56.3, U74.D7
- new net SDI: J6.DO/DAT0, Q10.3, R49.1, U8.~D22, U8.~D6
- new net SDI1: J17.DO/DAT0, Q11.3, R34.1, U6.~D22, U6.~D6
- new net SDI10: J98.DO/DAT0, Q65.3, R258.1, U82.~D22, U82.~D6
- new net SDI11: J107.DO/DAT0, Q71.3, R282.1, U90.~D22, U90.~D6
- new net SDI12: J116.DO/DAT0, Q77.3, R306.1, U98.~D22, U98.~D6
- new net SDI13: J125.DO/DAT0, Q83.3, R330.1, U106.~D22, U106.~D6
- new net SDI14: J134.DO/DAT0, Q89.3, R354.1, U114.~D22, U114.~D6
- new net SDI2: J26.DO/DAT0, Q17.3, R66.1, U18.~D22, U18.~D6
- new net SDI3: J35.DO/DAT0, Q23.3, R90.1, U26.~D22, U26.~D6
- new net SDI4: J44.DO/DAT0, Q29.3, R114.1, U34.~D22, U34.~D6
- new net SDI5: J53.DO/DAT0, Q35.3, R138.1, U42.~D22, U42.~D6
- new net SDI6: J62.DO/DAT0, Q41.3, R162.1, U50.~D22, U50.~D6
- new net SDI7: J71.DO/DAT0, Q47.3, R186.1, U58.~D22, U58.~D6
- new net SDI8: J80.DO/DAT0, Q53.3, R210.1, U66.~D22, U66.~D6
- new net SDI9: J89.DO/DAT0, Q59.3, R234.1, U74.~D22, U74.~D6
- new net SDO: J6.DI/CMD, Q3.3, U8.D7
- new net SDO1: J17.DI/CMD, Q5.3, U6.D7
- new net SDO10: J98.DI/CMD, Q62.3, U82.D7
- new net SDO11: J107.DI/CMD, Q68.3, U90.D7
- new net SDO12: J116.DI/CMD, Q74.3, U98.D7
- new net SDO13: J125.DI/CMD, Q80.3, U106.D7
- new net SDO14: J134.DI/CMD, Q86.3, U114.D7
- new net SDO2: J26.DI/CMD, Q14.3, U18.D7
- new net SDO3: J35.DI/CMD, Q20.3, U26.D7
- new net SDO4: J44.DI/CMD, Q26.3, U34.D7
- new net SDO5: J53.DI/CMD, Q32.3, U42.D7
- new net SDO6: J62.DI/CMD, Q38.3, U50.D7
- new net SDO7: J71.DI/CMD, Q44.3, U58.D7
- new net SDO8: J80.DI/CMD, Q50.3, U66.D7
- new net SDO9: J89.DI/CMD, Q56.3, U74.D7
- net DAT1: now also J6.DAT1; no longer J6.RSV2
- net DAT10: now also J44.DAT2; no longer J44.RSV1
- net DAT11: now also J53.DAT1; no longer J53.RSV2
- net DAT12: now also J53.DAT2; no longer J53.RSV1
- net DAT13: now also J62.DAT1; no longer J62.RSV2
- net DAT14: now also J62.DAT2; no longer J62.RSV1
- net DAT15: now also J71.DAT1; no longer J71.RSV2
- net DAT16: now also J71.DAT2; no longer J71.RSV1
- net DAT17: now also J80.DAT1; no longer J80.RSV2
- net DAT18: now also J80.DAT2; no longer J80.RSV1
- net DAT19: now also J89.DAT1; no longer J89.RSV2
- net DAT2: now also J6.DAT2; no longer J6.RSV1
- net DAT20: now also J89.DAT2; no longer J89.RSV1
- net DAT21: now also J98.DAT1; no longer J98.RSV2
- net DAT22: now also J98.DAT2; no longer J98.RSV1
- net DAT23: now also J107.DAT1; no longer J107.RSV2
- net DAT24: now also J107.DAT2; no longer J107.RSV1
- net DAT25: now also J116.DAT1; no longer J116.RSV2
- net DAT26: now also J116.DAT2; no longer J116.RSV1
- net DAT27: now also J125.DAT1; no longer J125.RSV2
- net DAT28: now also J125.DAT2; no longer J125.RSV1
- net DAT29: now also J134.DAT1; no longer J134.RSV2
- net DAT3: now also J17.DAT1; no longer J17.RSV2
- net DAT30: now also J134.DAT2; no longer J134.RSV1
- net DAT4: now also J17.DAT2; no longer J17.RSV1
- net DAT5: now also J26.DAT1; no longer J26.RSV2
- net DAT6: now also J26.DAT2; no longer J26.RSV1
- net DAT7: now also J35.DAT1; no longer J35.RSV2
- net DAT8: now also J35.DAT2; no longer J35.RSV1
- net DAT9: now also J44.DAT1; no longer J44.RSV2
- net GND: now also GND.P$1
- net GND1: now also GND1.P$1
- net GND10: now also GND10.P$1
- net GND11: now also GND11.P$1
- net GND12: now also GND12.P$1
- net GND13: now also GND13.P$1
- net GND14: now also GND14.P$1
- net GND2: now also GND2.P$1
- net GND3: now also GND3.P$1
- net GND4: now also GND4.P$1
- net GND5: now also GND5.P$1
- net GND6: now also GND6.P$1
- net GND7: now also GND7.P$1
- net GND8: now also GND8.P$1
- net GND9: now also GND9.P$1
- net MICROSD_!CS!: now also J6.CS/DAT3; no longer J6.CS
- net MICROSD_!CS!1: now also J17.CS/DAT3; no longer J17.CS
- net MICROSD_!CS!10: now also J98.CS/DAT3; no longer J98.CS
- net MICROSD_!CS!11: now also J107.CS/DAT3; no longer J107.CS
- net MICROSD_!CS!12: now also J116.CS/DAT3; no longer J116.CS
- net MICROSD_!CS!13: now also J125.CS/DAT3; no longer J125.CS
- net MICROSD_!CS!14: now also J134.CS/DAT3; no longer J134.CS
- net MICROSD_!CS!2: now also J26.CS/DAT3; no longer J26.CS
- net MICROSD_!CS!3: now also J35.CS/DAT3; no longer J35.CS
- net MICROSD_!CS!4: now also J44.CS/DAT3; no longer J44.CS
- net MICROSD_!CS!5: now also J53.CS/DAT3; no longer J53.CS
- net MICROSD_!CS!6: now also J62.CS/DAT3; no longer J62.CS
- net MICROSD_!CS!7: now also J71.CS/DAT3; no longer J71.CS
- net MICROSD_!CS!8: now also J80.CS/DAT3; no longer J80.CS
- net MICROSD_!CS!9: now also J89.CS/DAT3; no longer J89.CS
- net QWIIC_3.3V: now also QWIIC_3.3V.P$1
- net QWIIC_3.3V1: now also QWIIC_3.3V1.P$1
- net QWIIC_3.3V10: now also QWIIC_3.3V10.P$1
- net QWIIC_3.3V11: now also QWIIC_3.3V11.P$1
- net QWIIC_3.3V12: now also QWIIC_3.3V12.P$1
- net QWIIC_3.3V13: now also QWIIC_3.3V13.P$1
- net QWIIC_3.3V14: now also QWIIC_3.3V14.P$1
- net QWIIC_3.3V2: now also QWIIC_3.3V2.P$1
- net QWIIC_3.3V3: now also QWIIC_3.3V3.P$1
- net QWIIC_3.3V4: now also QWIIC_3.3V4.P$1
- net QWIIC_3.3V5: now also QWIIC_3.3V5.P$1
- net QWIIC_3.3V6: now also QWIIC_3.3V6.P$1
- net QWIIC_3.3V7: now also QWIIC_3.3V7.P$1
- net QWIIC_3.3V8: now also QWIIC_3.3V8.P$1
- net QWIIC_3.3V9: now also QWIIC_3.3V9.P$1
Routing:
- net SDI3: track 0.00 -> 50.4 mm, vias 0 -> 2
- net MISO3: track 50.4 -> 0.00 mm, vias 2 -> 0
- net SDI4: track 0.00 -> 50.4 mm, vias 0 -> 2
- net MISO4: track 50.4 -> 0.00 mm, vias 2 -> 0
- net SDI7: track 0.00 -> 50.4 mm, vias 0 -> 2
- net SDI6: track 0.00 -> 50.4 mm, vias 0 -> 2
- net SDI1: track 0.00 -> 50.4 mm, vias 0 -> 2
- net MISO7: track 50.4 -> 0.00 mm, vias 2 -> 0
- net MISO6: track 50.4 -> 0.00 mm, vias 2 -> 0
- net MISO1: track 50.4 -> 0.00 mm, vias 2 -> 0
- net SDI: track 0.00 -> 50.4 mm, vias 0 -> 2
- net MISO: track 50.4 -> 0.00 mm, vias 2 -> 0
- net SDI5: track 0.00 -> 50.4 mm, vias 0 -> 2
- net MISO5: track 50.4 -> 0.00 mm, vias 2 -> 0
- net SDI8: track 0.00 -> 50.4 mm, vias 0 -> 2
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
